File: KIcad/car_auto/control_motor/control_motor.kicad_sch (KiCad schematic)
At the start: 8 parts, among them J1 B6P-VH_LF__SN_, J2 B2P-VH_LF__SN_, U1 YAAJ_DCDC_StepDown_LM2596, U2 L298N DUAL H-BRIDGE MOTOR DRI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

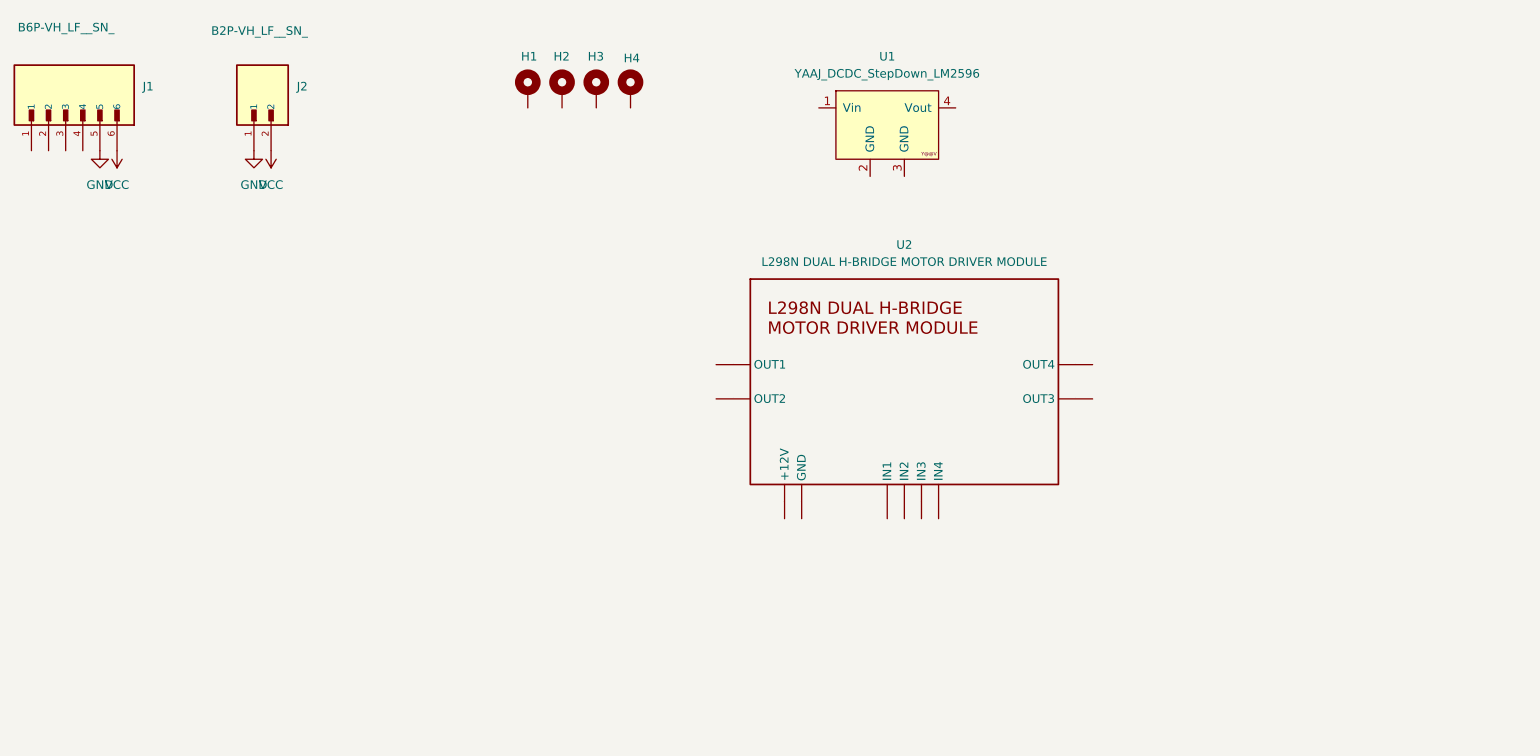
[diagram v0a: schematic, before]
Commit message: feat: Implementação da classe para controle dos motores via Bluetooth.
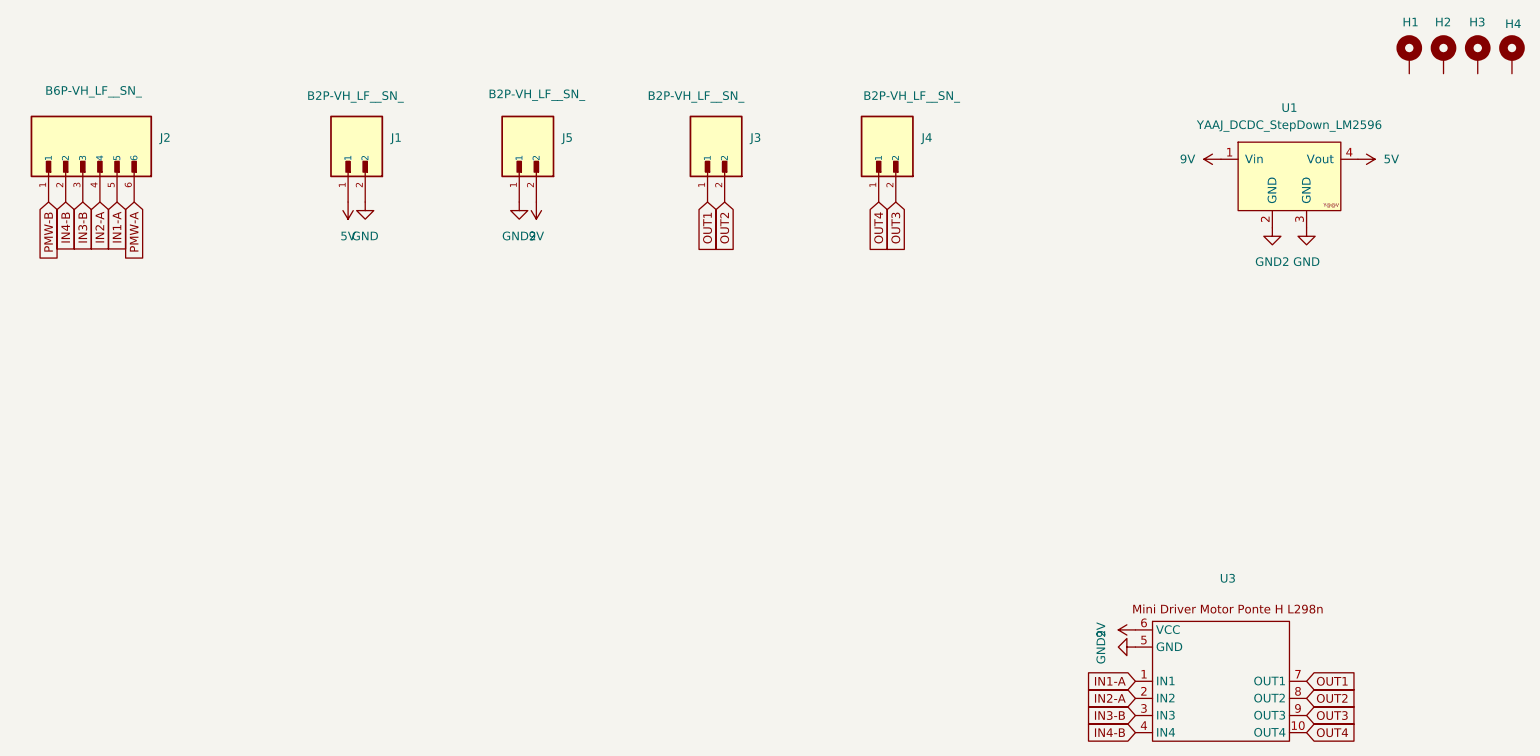
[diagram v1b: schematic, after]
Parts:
- removed J1: B6P-VH_LF__SN_, importados:JST_B6P-VH_LF__SN_, symbol importados:B6P-VH_LF__SN_
- removed J2: B2P-VH_LF__SN_, importados:JST_B2P-VH_LF__SN_, symbol importados:B2P-VH_LF__SN_
- removed U2: L298N DUAL H-BRIDGE MOTOR DRIVER MODULE, importados:L298N DUAL H-BRIDGE MOTOR DRIVER MODULE FOOTPRINT, symbol importados:L298N DUAL H-BRIDGE MOTOR DRIVER MODULE
- added J1, J3, J4, J5: B2P-VH_LF__SN_, importados:JST_B2P-VH_LF__SN_, symbol importados:B2P-VH_LF__SN_
- added J2: B6P-VH_LF__SN_, importados:JST_B6P-VH_LF__SN_, symbol importados:B6P-VH_LF__SN_
- added U3: ~, importados:Mini Driver Motor Ponte H L298n, symbol importados:Mini_L298N
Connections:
- net GND: now also U1.3 (GND), J1.2
- net 9V: now reaches U1.1 (Vin)
- net 9V: now also J5.2, U3.6 (VCC)
- net GND2: now reaches U1.2 (GND)
- net GND2: now also J5.1, U3.5 (GND)
- net 5V: now reaches U1.4 (Vout)
- net 5V: now also J1.1
- new net IN1-A: J2.5, U3.1 (IN1)
- new net IN2-A: J2.4, U3.2 (IN2)
- new net IN3-B: J2.3, U3.3 (IN3)
- new net IN4-B: J2.2, U3.4 (IN4)
- new net OUT1: J3.1, U3.7 (OUT1)
- new net OUT2: J3.2, U3.8 (OUT2)
- new net OUT3: J4.2, U3.9 (OUT3)
- new net OUT4: J4.1, U3.10 (OUT4)
- new net PMW-A: J2.6
- new net PMW-B: J2.1
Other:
- moved on the sheet: U1
